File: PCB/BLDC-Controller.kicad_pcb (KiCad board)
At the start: 2 copper layers, 24 x 45.2 mm, 47 parts, among them J1 Mot_Con, J10 Receiver, J2 Mot_Con, J3 Mot_Con, J4 Mot_Con, J5 Mot_Con, J6 Mot_Con, J7 Bat+, J8 Bat-, J9 Prog, Q1 P75NF75, Q2 P75NF75, Q3 P75NF75, Q4 P75NF75, Q5 P75NF75, Q6 P75NF75, U1 UCC27282, U2 UCC27282, U3 UCC27282, U4 ATmega328P-A, Y1 16M

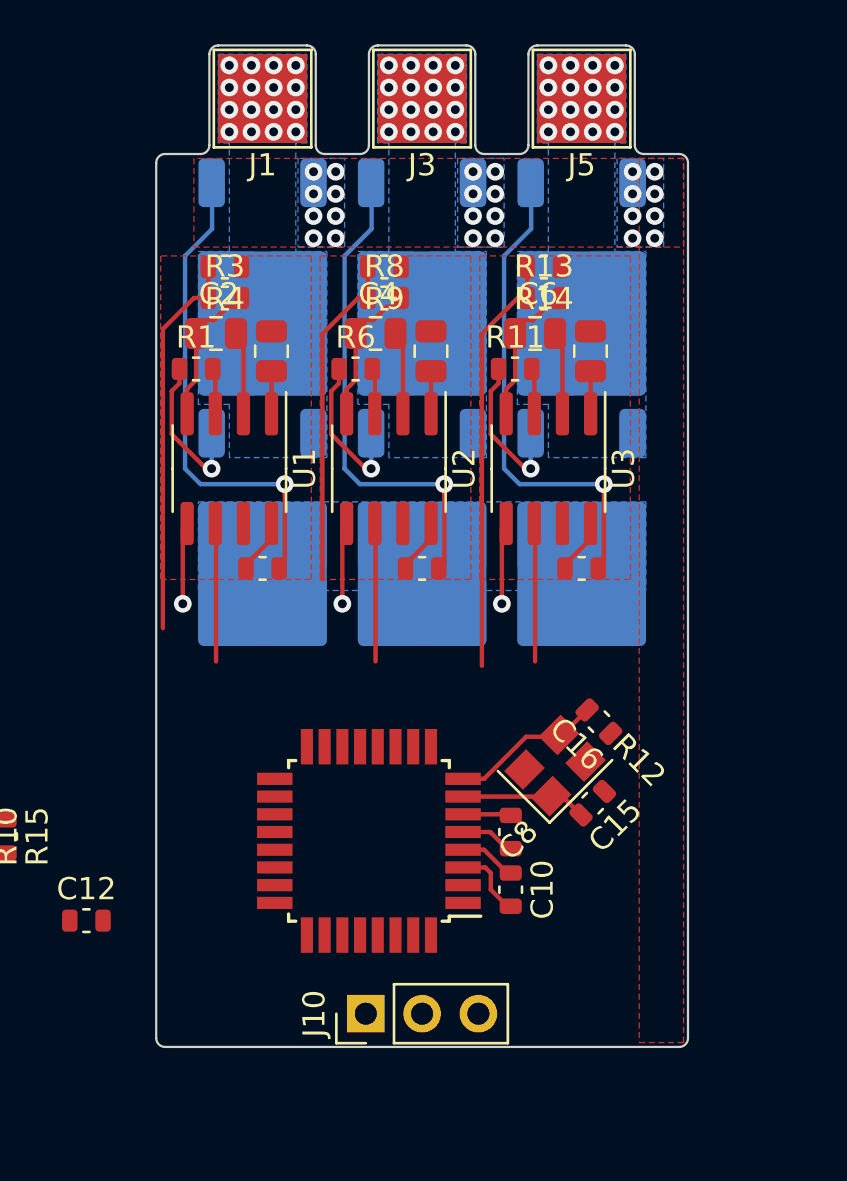
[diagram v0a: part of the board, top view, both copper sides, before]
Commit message: k
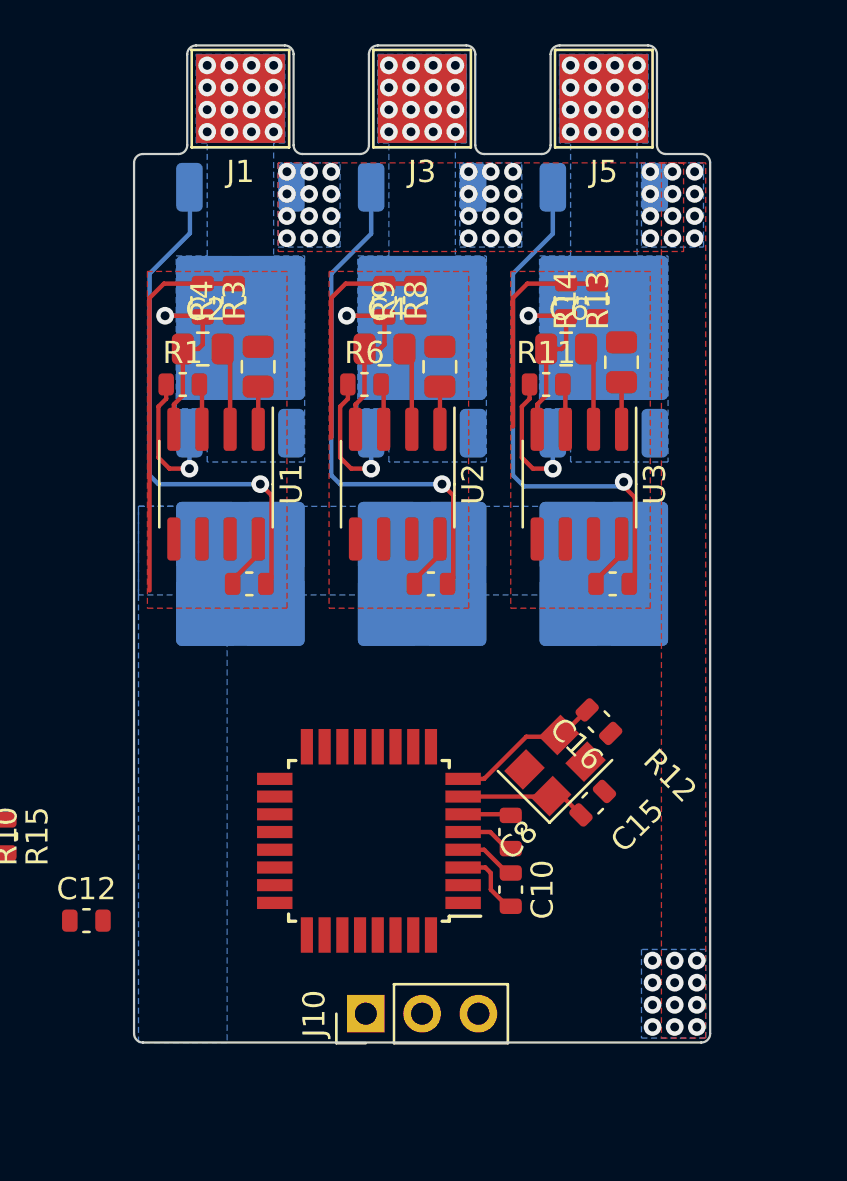
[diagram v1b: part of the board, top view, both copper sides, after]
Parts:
- moved R14 2.83 mm to (81.9, 39.0), turned to 90 degrees
- moved R9 2.05 mm to (73.7, 39.0), turned to 90 degrees
- moved C6 1.57 mm to (80.5, 41.2)
- moved R11 1.57 mm to (79.6, 42.8)
- moved R12 1.57 mm to (82.6, 51.8)
- moved U3 1.57 mm to (81.1, 47.3)
- moved R4 1.55 mm to (65.5, 39.0), turned to 90 degrees
- moved C5 1.49 mm to (83.0, 41.8)
- moved Q2 1.02 mm to (65.8, 39.0)
- moved Q6 1.02 mm to (82.2, 39.0)
- moved R13 1.00 mm to (80.5, 39.0), turned to -90 degrees
- moved R3 1.00 mm to (64.1, 39.0), turned to -90 degrees
- moved J1 1.00 mm to (65.8, 29.9)
- moved J2 1.00 mm to (65.8, 29.9)
- moved J5 1.00 mm to (82.2, 29.9)
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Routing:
- net /MCU/V_Sen_C: track 19.1 -> 9.87 mm
- net /MCU/LI_C: track 6.19 -> 0.00 mm
- net /MCU/LI_B: track 6.19 -> 0.00 mm
- net /MCU/LI_A: track 6.19 -> 0.00 mm
- net /MCU/V_Sen_B: track 15.2 -> 10.4 mm
- net /MCU/HI_C: track 3.42 -> 0.00 mm, vias 1 -> 0
- net /MCU/HI_B: track 3.42 -> 0.00 mm, vias 1 -> 0
- net /MCU/HI_A: track 3.42 -> 0.00 mm, vias 1 -> 0
- net /Phase C/Phase_Out: track 6.04 -> 9.31 mm, vias 16 -> 17
- net /Phase A/Phase_Out: track 6.04 -> 9.21 mm, vias 16 -> 17
- net /Phase B/Phase_Out: track 6.04 -> 9.20 mm, vias 16 -> 17
- net Net-(Q4-G): track 21.7 -> 23.4 mm
- net Net-(Q2-G): track 21.7 -> 23.3 mm
- net Net-(Q6-G): track 21.7 -> 23.3 mm
- net GND: vias 24 -> 48
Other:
- board size 24 x 45.2 mm -> 26 x 45 mm
